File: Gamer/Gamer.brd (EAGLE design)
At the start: 162 x 64 mm, 53 parts, among them J1 AVR_SPI_PRG_6NS, J2 AVR_SPI_PRG_6NS, J3 AVR_SPI_PRG_6NS, J4 AVR_SPI_PRG_6NS

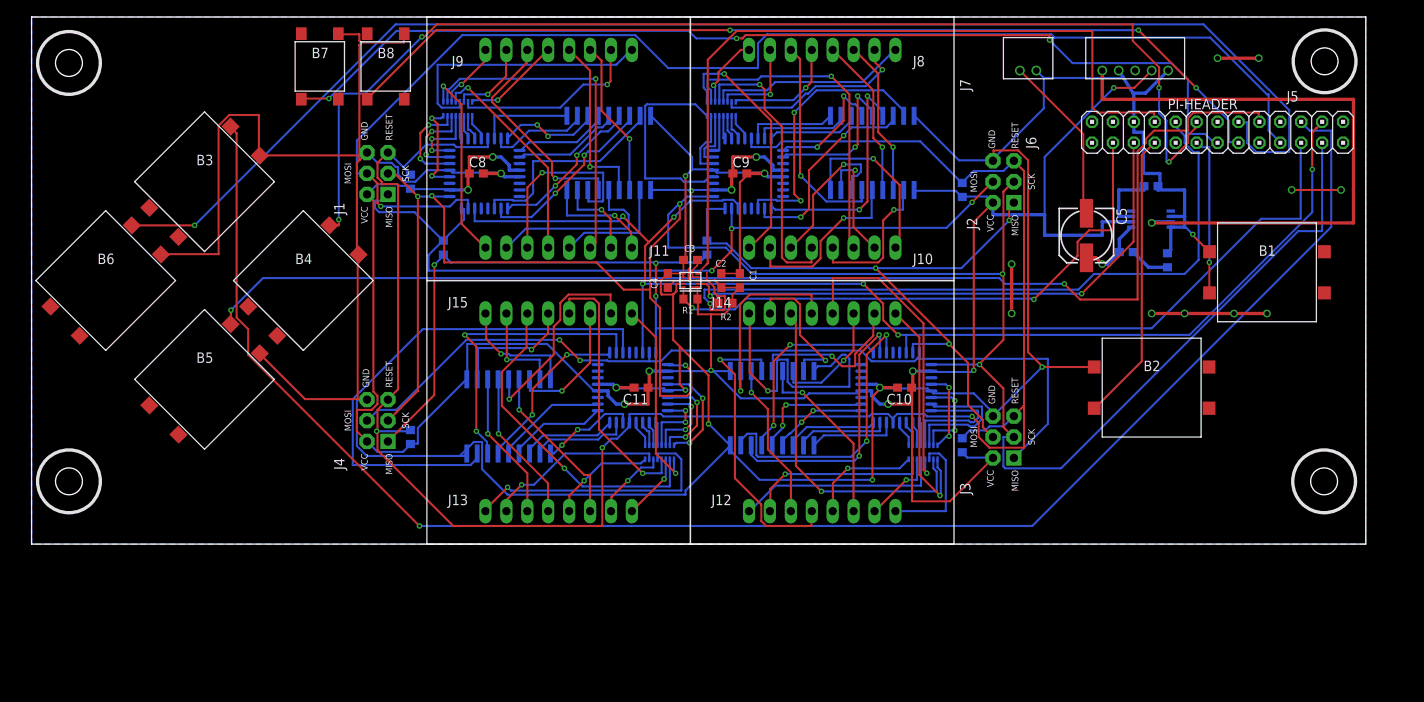
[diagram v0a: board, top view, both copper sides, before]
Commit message: gamer - Starting complete redo of Gamer
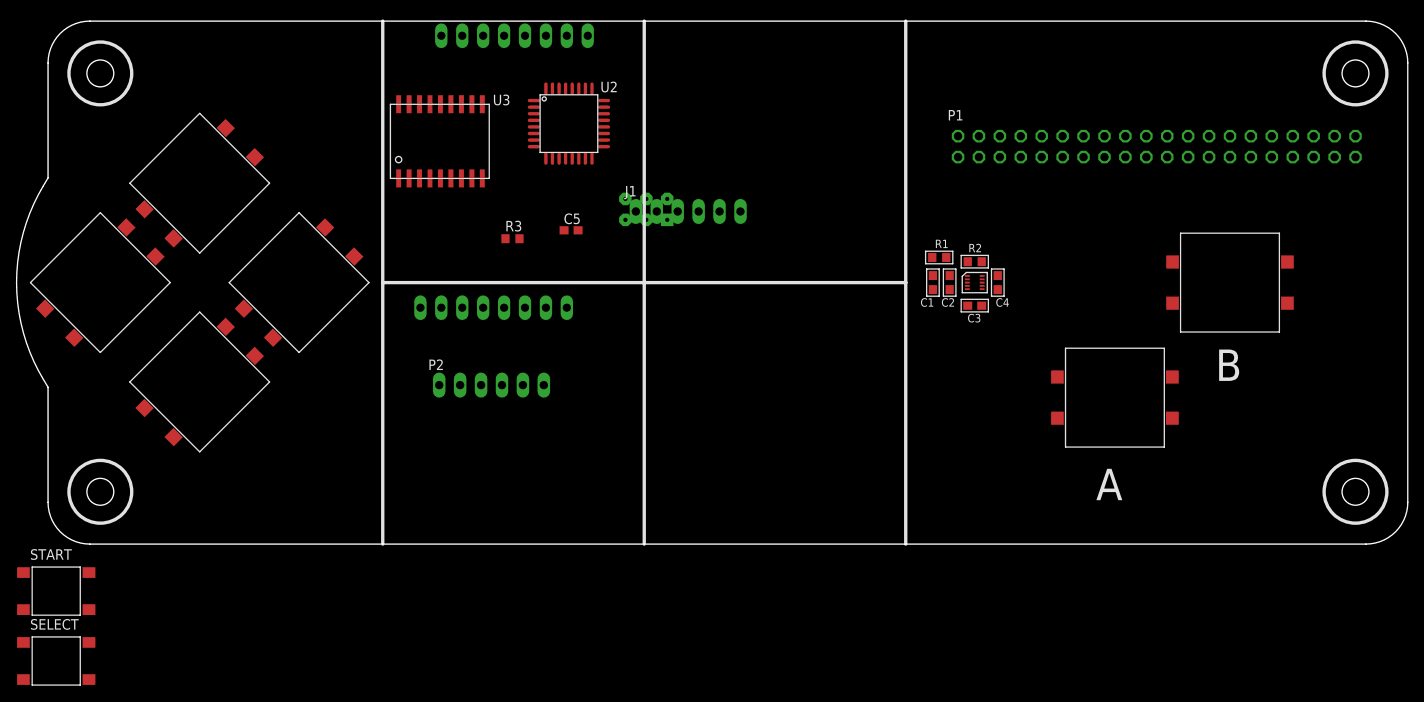
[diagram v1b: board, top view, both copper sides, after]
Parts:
- removed C10, C11, C8, C9: (no value), resistor:C0603
- removed C6: 0.05uF, resistor:C0603
- removed C7: 1uF, resistor:C0603
- removed J4: AVR_SPI_PRG_6NS, SparkFun-Connectors:2X3-NS
- removed PI-HEADER: (no value), pinhead:2X13
- removed R4: Bypass, resistor:R0603
- removed R5, R6, R8, R9: 100K, resistor:R0603
- removed R7: 10, resistor:R0603
- removed U$1, U$13, U$3, U$8: 8X8_LED_MATRIX, ScottSilver:8X8_LED_MATRIX
- removed U$10, U$14, U$4, U$5: ULN2803AFWG, ScottSilver:ULN2803AFWG
- removed U$11, U$15, U$6, U$9: ATTINY48, ScottSilver:ATTINY48
- removed U$12, U$16, U$2, U$7: RES_ARRAY, ScottSilver:RES_ARRAY
- removed U$17, U$18, U$19, U$20, U$21, U$22: 12X12MM_BUTTON, ScottSilver:12X12MM_BUTTON
- removed U$23: MMA8653FCR1, ScottSilver:MMA8653FCR1
- removed U$24, U$26: SMDTACTILE, ScottSilver:SMDTACTILE
- removed U$25: LM386, ScottSilver:LM386
- removed U$29: DF3_1X2, ScottSilver:DF3_1X2
- removed U$30: DF3_1X5, ScottSilver:DF3_1X5
- added A, B, DOWN, LEFT, RIGHT, UP: 12X12MM_BUTTON, Gamer:12X12MM_BUTTON
- added P1: (no value), HeaderConnectorBoard:2X20
- added P2: NONE, LED_Matrix:1X06
- added PROG: NONE, LED_Matrix:2X03
- added SELECT, START: 6X6MM_BUTTON, Gamer:6X6MM_BUTTON
- added U1: MMA8653FCR1, AccelBreakout:MMA8653FCR1
- added U2: ATTINY48, LED_Matrix:ATTINY48
- added U3: ULN2803AFWG, LED_Matrix:ULN2803AFWG
- C1, C2, C3, C4: device resistor:C0603 -> AccelBreakout:C0603
- C5: value (none) -> 1uF; device resistor:153CLV-0605 -> resistor:C0603
- J1: value AVR_SPI_PRG_6NS -> NONE; device SparkFun-Connectors:2X3-NS -> LED_Matrix:1X06
- J2, J3: value AVR_SPI_PRG_6NS -> HEADER-1X8; device SparkFun-Connectors:2X3-NS -> LED_Matrix:HEADER-1X8
- R1, R2: value 1k -> 10K; device resistor:R0603 -> AccelBreakout:R0603
- R3: value Bypass -> 10k
- moved J2 63.8 mm to (54.1, 28.7), turned to 0 degrees
- moved C5 62.6 mm to (63.5, 38.1), turned to 0 degrees
- moved J3 49.6 mm to (56.6, 61.7), turned to 0 degrees
- moved C4 40.1 mm to (115.3, 31.8), turned to 270 degrees
- moved J1 38.0 mm to (77.7, 40.4), turned to 0 degrees
- moved C3 35.0 mm to (112.5, 29.0), turned to 0 degrees
- moved R2 30.7 mm to (112.5, 34.3)
- moved R1 30.6 mm to (108.2, 34.8), turned to 180 degrees
- moved C2 27.7 mm to (109.5, 31.8), turned to 270 degrees
- moved C1 23.4 mm to (107.4, 31.8), turned to 270 degrees
- moved R3 8.46 mm to (56.4, 37.1), flipped to the top, turned to 0 degrees
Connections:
- removed net A: PI-HEADER.7, U$22.3
- removed net AUDIO: U$25.3, U$30.1
- removed net B: PI-HEADER.11, U$21.3
- removed net DOWN: PI-HEADER.18, U$20.2
- removed net LEFT: PI-HEADER.16, U$18.2
- removed net MISO1/MOSI2: J1.1, J2.4, R3.1, U$6.PB3, U$9.PB4
- removed net MISO2/MOSI3: J2.1, J4.4, R4.1, U$15.PB3, U$6.PB4
- removed net MISO3/MOSI4: J3.4, J4.1, U$11.PB3, U$15.PB4
- removed net N$1: U$1.COL0, U$5.O1
- removed net N$10: U$1.ROW6, U$2.2R
- removed net N$100: U$11.PC4, U$12.R2
- removed net N$101: U$11.PC5, U$12.R1
- removed net N$102: U$15.PC7, U$16.R8
- removed net N$103: U$13.COL0, U$14.O1
- removed net N$104: U$13.COL1, U$14.O2
- removed net N$105: U$13.COL2, U$14.O3
- removed net N$106: U$13.COL3, U$14.O4
- removed net N$107: U$13.COL4, U$14.O5
- removed net N$108: U$13.COL5, U$14.O6
- removed net N$109: U$13.COL6, U$14.O7
- removed net N$11: U$1.ROW5, U$2.3R
- removed net N$110: U$13.COL7, U$14.O8
- removed net N$111: U$13.ROW7, U$16.1R
- removed net N$112: U$13.ROW6, U$16.2R
- removed net N$113: U$13.ROW5, U$16.3R
- removed net N$114: U$13.ROW4, U$16.4R
- removed net N$115: U$13.ROW3, U$16.5R
- removed net N$116: U$13.ROW2, U$16.6R
- removed net N$117: U$13.ROW1, U$16.7R
- removed net N$118: U$13.ROW0, U$16.8R
- removed net N$119: U$14.I1, U$15.PD0
- removed net N$12: U$1.ROW4, U$2.4R
- removed net N$120: U$14.I2, U$15.PD1
- removed net N$121: U$14.I3, U$15.PD2
- removed net N$122: U$14.I4, U$15.PD3
- removed net N$123: U$14.I5, U$15.PD4
- removed net N$124: U$14.I6, U$15.PD5
- removed net N$125: U$14.I7, U$15.PD6
- removed net N$126: U$14.I8, U$15.PD7
- removed net N$129: U$15.PC0, U$16.R6
- removed net N$13: U$1.ROW3, U$2.5R
- removed net N$130: U$15.PC1, U$16.R5
- removed net N$131: U$15.PC2, U$16.R4
- removed net N$132: U$15.PC3, U$16.R3
- removed net N$133: U$15.PC4, U$16.R2
- removed net N$134: U$15.PC5, U$16.R1
- removed net N$14: U$1.ROW2, U$2.6R
- removed net N$15: U$1.ROW1, U$2.7R
- removed net N$16: U$1.ROW0, U$2.8R
- removed net N$17: U$5.I1, U$9.PD0
- removed net N$18: U$5.I2, U$9.PD1
- removed net N$19: U$5.I3, U$9.PD2
- removed net N$2: U$1.COL1, U$5.O2
- removed net N$20: U$5.I4, U$9.PD3
- removed net N$21: U$5.I5, U$9.PD4
- removed net N$22: U$5.I6, U$9.PD5
- removed net N$23: U$5.I7, U$9.PD6
- removed net N$24: U$5.I8, U$9.PD7
- removed net N$25: U$2.R7, U$9.PA1
- removed net N$26: U$2.R8, U$9.PC7
- removed net N$27: U$2.R6, U$9.PC0
- removed net N$28: U$2.R5, U$9.PC1
- removed net N$29: U$2.R4, U$9.PC2
- removed net N$3: U$1.COL2, U$5.O3
- removed net N$30: U$2.R3, U$9.PC3
- removed net N$31: U$2.R2, U$9.PC4
- removed net N$32: U$2.R1, U$9.PC5
- removed net N$33: C7.1, U$25.7
- removed net N$35: C5.+, C6.1, U$25.5
- removed net N$36: U$3.COL0, U$4.O1
- removed net N$37: C6.2, R7.2
- removed net N$38: U$3.COL1, U$4.O2
- removed net N$39: U$3.COL2, U$4.O3
- removed net N$4: U$1.COL3, U$5.O4
- removed net N$40: U$3.COL3, U$4.O4
- removed net N$41: U$3.COL4, U$4.O5
- removed net N$42: U$3.COL5, U$4.O6
- removed net N$43: U$3.COL6, U$4.O7
- removed net N$44: U$3.COL7, U$4.O8
- removed net N$45: U$3.ROW7, U$7.1R
- removed net N$46: U$3.ROW6, U$7.2R
- removed net N$47: U$3.ROW5, U$7.3R
- removed net N$48: U$3.ROW4, U$7.4R
- removed net N$49: U$3.ROW3, U$7.5R
- removed net N$5: U$1.COL4, U$5.O5
- removed net N$50: U$3.ROW2, U$7.6R
- removed net N$51: U$3.ROW1, U$7.7R
- removed net N$52: U$3.ROW0, U$7.8R
- removed net N$53: U$4.I1, U$6.PD0
- removed net N$54: U$4.I2, U$6.PD1
- removed net N$55: U$4.I3, U$6.PD2
- removed net N$56: U$4.I4, U$6.PD3
- removed net N$57: U$4.I5, U$6.PD4
- removed net N$58: U$4.I6, U$6.PD5
- removed net N$59: U$4.I7, U$6.PD6
- removed net N$6: U$1.COL5, U$5.O6
- removed net N$60: U$4.I8, U$6.PD7
- removed net N$61: U$6.PA1, U$7.R7
- removed net N$62: U$6.PC7, U$7.R8
- removed net N$63: U$6.PC0, U$7.R6
- removed net N$64: U$6.PC1, U$7.R5
- removed net N$65: U$6.PC2, U$7.R4
- removed net N$66: U$6.PC3, U$7.R3
- removed net N$67: U$6.PC4, U$7.R2
- removed net N$68: U$6.PC5, U$7.R1
- removed net N$69: U$15.PA1, U$16.R7
- removed net N$7: U$1.COL6, U$5.O7
- removed net N$70: U$10.O1, U$8.COL0
- removed net N$71: U$10.O2, U$8.COL1
- removed net N$72: U$10.O3, U$8.COL2
- removed net N$73: U$10.O4, U$8.COL3
- removed net N$74: U$10.O5, U$8.COL4
- removed net N$75: U$10.O6, U$8.COL5
- removed net N$76: U$10.O7, U$8.COL6
- removed net N$77: U$10.O8, U$8.COL7
- removed net N$78: U$12.1R, U$8.ROW7
- removed net N$79: U$12.2R, U$8.ROW6
- removed net N$8: U$1.COL7, U$5.O8
- removed net N$80: U$12.3R, U$8.ROW5
- removed net N$81: U$12.4R, U$8.ROW4
- removed net N$82: U$12.5R, U$8.ROW3
- removed net N$83: U$12.6R, U$8.ROW2
- removed net N$84: U$12.7R, U$8.ROW1
- removed net N$85: U$12.8R, U$8.ROW0
- removed net N$86: U$10.I1, U$11.PD0
- removed net N$87: U$10.I2, U$11.PD1
- removed net N$88: U$10.I3, U$11.PD2
- removed net N$89: U$10.I4, U$11.PD3
- removed net N$9: U$1.ROW7, U$2.1R
- removed net N$90: U$10.I5, U$11.PD4
- removed net N$91: U$10.I6, U$11.PD5
- removed net N$92: U$10.I7, U$11.PD6
- removed net N$93: U$10.I8, U$11.PD7
- removed net N$94: U$11.PA1, U$12.R7
- removed net N$95: U$11.PC7, U$12.R8
- removed net N$96: U$11.PC0, U$12.R6
- removed net N$97: U$11.PC1, U$12.R5
- removed net N$98: U$11.PC2, U$12.R4
- removed net N$99: U$11.PC3, U$12.R3
- removed net RIGHT: PI-HEADER.12, U$19.2
- removed net SELECT: PI-HEADER.15, U$26.1
- removed net SPK: C5.-, U$29.1
- removed net SS: PI-HEADER.24, U$11.PB2, U$15.PB2, U$6.PB2, U$9.PB2
- removed net START: PI-HEADER.13, U$24.1
- removed net UP: PI-HEADER.22, U$17.2
- new net 10/MOSI: P1.19
- new net 11/CLK: P1.23
- new net 12: P1.32
- new net 13: P1.33
- new net 14/TX: P1.8
- new net 15/RX: P1.10
- new net 16: P1.36
- new net 17/RTS: B.3, P1.11
- new net 18: P1.12, RIGHT.2
- new net 19: P1.35
- new net 2/SDA: P1.3
- new net 20: P1.38
- new net 21: P1.40
- new net 22: P1.15, SELECT.2
- new net 23: LEFT.2, P1.16
- new net 24: DOWN.2, P1.18
- new net 25: P1.22, UP.2
- new net 26: P1.37
- new net 27: P1.13, START.2
- new net 3.3V_1: P1.1
- new net 3.3V_2: P1.17
- new net 3/SCL: P1.5
- new net 4: A.3, P1.7
- new net 5: P1.29
- new net 5V_1: P1.4
- new net 5V_2: P1.2
- new net 6: P1.31
- new net 7/CE1: P1.26
- new net 8/CE0: P1.24
- new net 9/MISO: P1.21
- new net COL0: J3.8, U3.O1
- new net COL0_SINK: U2.PD0, U3.I1
- new net COL1: J3.7, U3.O2
- new net COL1_SINK: U2.PD1, U3.I2
- new net COL2: J3.3, U3.O3
- new net COL2_SINK: U2.PD2, U3.I3
- new net COL3: J2.3, U3.O4
- new net COL3_SINK: U2.PD3, U3.I4
- new net COL4: J3.2, U3.O5
- new net COL4_SINK: U2.PD4, U3.I5
- new net COL5: J2.5, U3.O6
- new net COL5_SINK: U2.PD5, U3.I6
- new net COL6: J2.6, U3.O7
- new net COL6_SINK: U2.PD6, U3.I7
- new net COL7: J3.5, U3.O8
- new net COL7_SINK: U2.PD7, U3.I8
- new net CS: J1.4, P2.4, U2.PB2
- new net GND2: P1.25
- new net GND3: P1.20
- new net GND4: P1.14
- new net GND5: P1.6
- new net GND6: P1.39
- new net GND7: P1.34
- new net GND8: P1.30
- new net ID1: P1.27
- new net ID2: P1.28
- new net ROW0: J3.1, U2.PC7
- new net ROW1: J3.6, U2.PA1
- new net ROW2: J2.1, U2.PC0
- new net ROW3: J3.4, U2.PC1
- new net ROW4: J2.8, U2.PC2
- new net ROW5: J2.2, U2.PC3
- new net ROW6: J2.7, U2.PC4
- new net ROW7: J2.4, U2.PC5
- net GND: now also A.1, B.1, C5.2, DOWN.4, LEFT.4, P1.9, P2.6, PROG.2, RIGHT.4, SELECT.4, START.4, U1.6, U1.7, U1.9, U2.AGND, U2.GND, U3.GND, UP.4; no longer C10.2, C11.2, C7.2, C8.2, C9.2, J2.6, J3.6, J4.6, PI-HEADER.6, R7.1, U$10.GND, U$11.AGND, U$11.GND, U$14.GND, U$15.AGND, U$15.GND, U$17.4, U$18.4, U$19.4, U$20.4, U$21.1, U$22.1, U$23.6, U$23.7, U$23.9, U$24.4, U$25.2, U$25.4, U$26.4, U$29.2, U$30.2, U$30.5, U$4.GND, U$5.GND, U$6.AGND, U$6.GND, U$9.AGND, U$9.GND
- net INT1: now also U1.3; no longer PI-HEADER.10, U$23.3
- net INT2: now also U1.5; no longer PI-HEADER.8, U$23.5
- net MISO: now also J1.3, PROG.5, U2.PB4; no longer J3.1, PI-HEADER.21, R3.2, R4.2, U$11.PB4
- net MOSI: now also P2.3, PROG.4, U2.PB3; no longer J1.4, PI-HEADER.19, U$9.PB3
- net N$34: now also U1.4; no longer U$23.4
- net RESET: now also P2.5, PROG.1, R3.2, U2.PC6; no longer J2.5, J3.5, J4.5, R5.1, R6.1, R8.1, R9.1, U$11.PC6, U$15.PC6, U$6.PC6, U$9.PC6
- net SCK: now also J1.2, P2.2, PROG.3, U2.PB5; no longer J1.3, J2.3, J3.3, J4.3, PI-HEADER.23, U$11.PB5, U$15.PB5, U$6.PB5, U$9.PB5
- net SCL: now also R1.1, U1.2; no longer PI-HEADER.5, R2.2, U$23.2
- net SDA: now also R2.1, U1.10; no longer PI-HEADER.3, R1.1, U$23.10
- net VCC: now also C5.1, J1.1, P2.1, PROG.6, R2.2, R3.1, U1.1, U1.8, U2.AVCC, U2.VCC, U3.COMMON; no longer C10.1, C11.1, C8.1, C9.1, J1.2, J2.2, J3.2, J4.2, R2.1, R5.2, R6.2, R8.2, R9.2, U$10.COMMON, U$11.AVCC, U$11.VCC, U$14.COMMON, U$15.AVCC, U$15.VCC, U$23.1, U$23.8, U$25.6, U$30.4, U$4.COMMON, U$5.COMMON, U$6.AVCC, U$6.VCC, U$9.AVCC, U$9.VCC
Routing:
- net GND: track 509.6 -> 0.00 mm, vias 20 -> 0
- net VCC: track 321.8 -> 0.00 mm, vias 12 -> 0
- net SCK: track 266.7 -> 0.00 mm, vias 6 -> 0
- net RESET: track 240.3 -> 0.00 mm, vias 3 -> 0
- net UP: track 199.5 -> 0.00 mm, vias 1 -> 0
- net LEFT: track 169.2 -> 0.00 mm, vias 1 -> 0
- net MISO: track 162.3 -> 0.00 mm, vias 3 -> 0
- net SS: track 156.7 -> 0.00 mm, vias 6 -> 0
- net MOSI: track 152.5 -> 0.00 mm, vias 1 -> 0
- net DOWN: track 151.5 -> 0.00 mm, vias 2 -> 0
- net RIGHT: track 142.0 -> 0.00 mm, vias 4 -> 0
- net START: track 124.9 -> 0.00 mm, vias 3 -> 0
- net SELECT: track 116.5 -> 0.00 mm, vias 3 -> 0
- net MISO3/MOSI4: track 104.7 -> 0.00 mm, vias 2 -> 0
- net MISO1/MOSI2: track 99.5 -> 0.00 mm, vias 3 -> 0
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- removed copper zone on layer 16, net GND
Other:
- board size 162 x 64 mm -> 168.9 x 63.5 mm
- board text removed: "B1"
- board text removed: "B2"
- board text removed: "B3"
- board text removed: "B4"
- board text removed: "B5"
- board text removed: "B6"
- board text removed: "B7"
- board text removed: "B8"
- board text removed: "GND"
- board text removed: "J1"
- board text removed: "J10"
- board text removed: "J11"
- board text removed: "J12"
- board text removed: "J13"
- board text removed: "J14"
- board text removed: "J15"
- board text removed: "J3"
- board text removed: "J4"
- board text removed: "J5"
- board text removed: "J6"
- board text removed: "J7"
- board text removed: "J8"
- board text removed: "J9"
- board text removed: "MISO"
- board text removed: "MOSI"
- board text removed: "RESET"
- board text removed: "SCK"
- board text removed: "U1"
- board text removed: "U2"
- board text removed: "U3"
- board text removed: "U4"
- board text removed: "U5"
- board text removed: "U6"
- board text removed: "U7"
- board text removed: "U8"
- board text removed: "VCC"
